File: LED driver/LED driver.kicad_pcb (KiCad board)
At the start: 2 copper layers, 50 x 40 mm, 42 parts, among them J1 Conn_VCC, J2 Conn_LED, J3 Conn_Aux, J4 Conn_UART, Q1 ZXMN3A01F, Q2 ZXMN3A01F, Q3 ZXMN3A01F, Q4 ZXMN3A01F, Q5 ZXMN3A01F, SW1 SW_Push, U1 ESP32-C3-MINI-1-N4, U2 MP2359

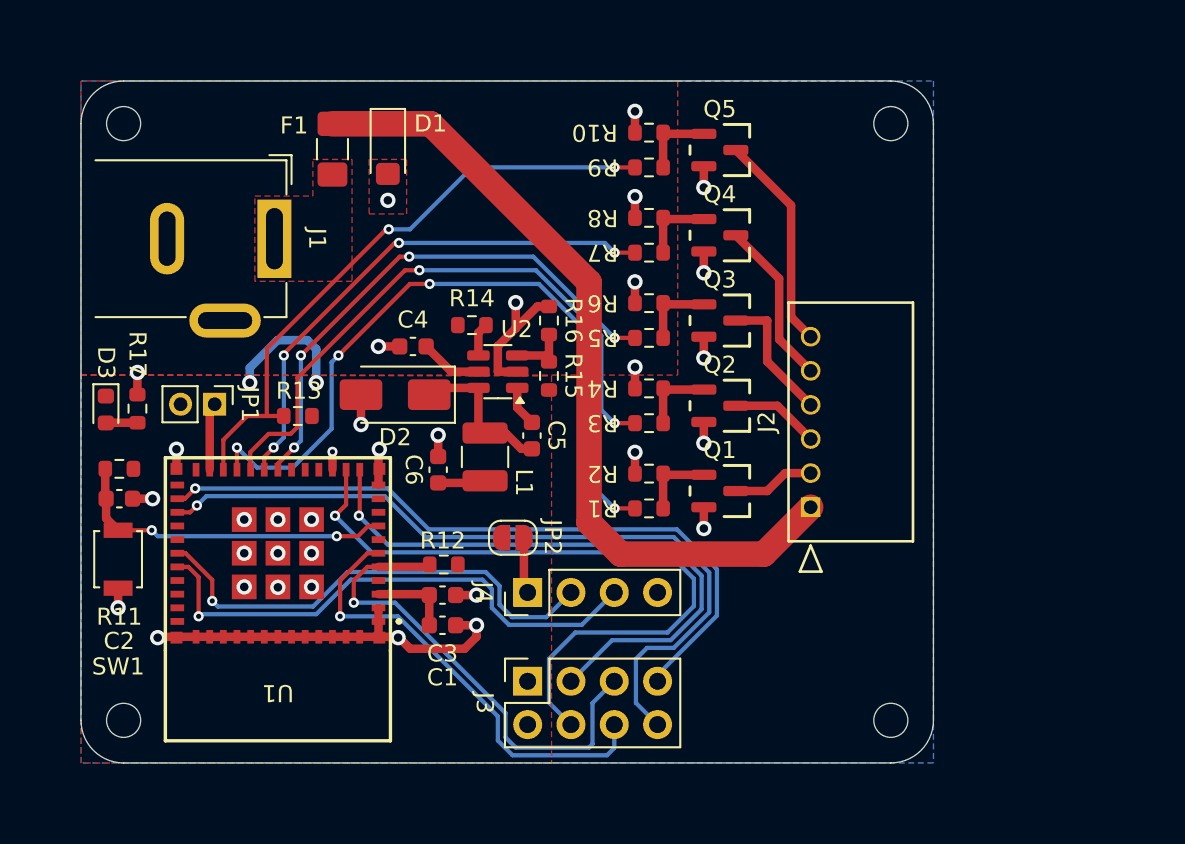
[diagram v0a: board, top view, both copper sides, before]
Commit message: 2024-06-04 002
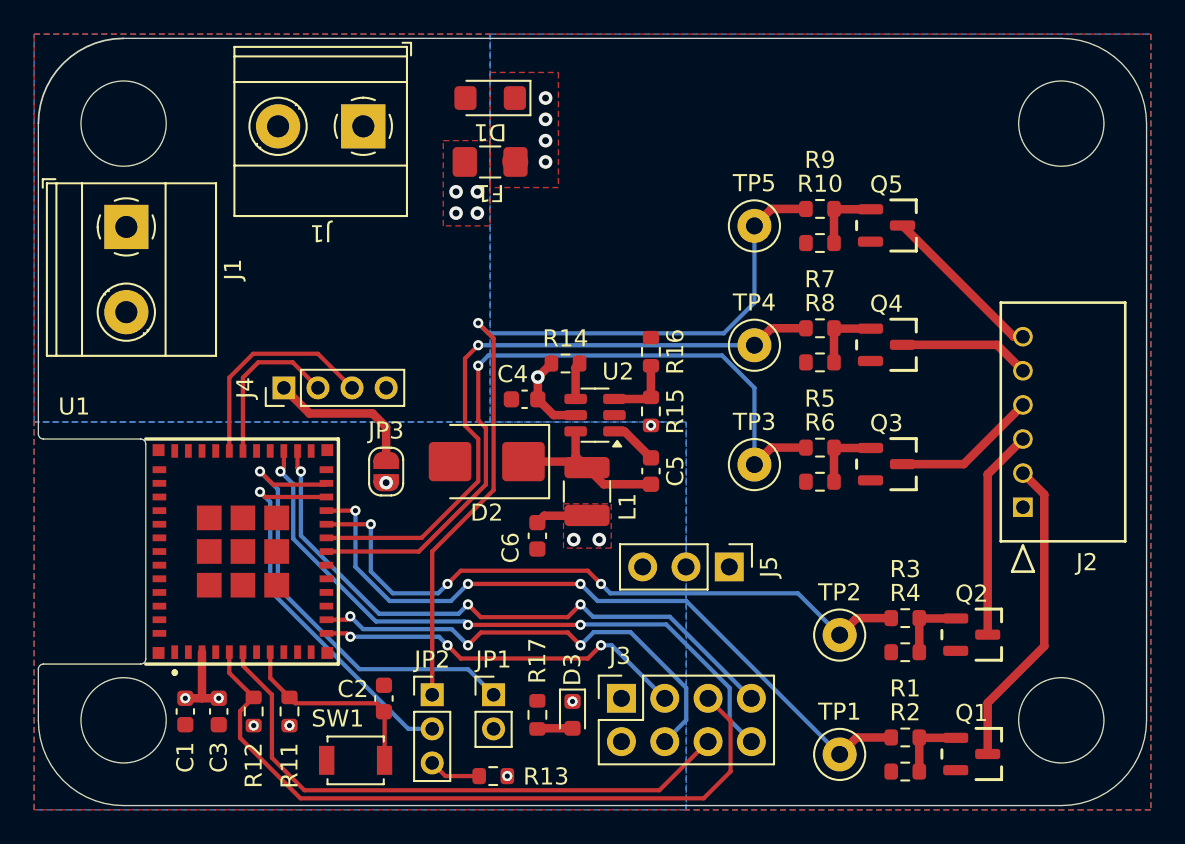
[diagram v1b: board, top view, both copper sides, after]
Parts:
- removed the J1 at (108.7, 64.3)
- added J1: Conn_VCC, TerminalBlock_Phoenix:TerminalBlock_Phoenix_MKDS-1,5-2_1x02_P5.00mm_Horizontal, F.Cu at (113.9, 57.7)
- added J1: Conn_VCC, TerminalBlock_Phoenix:TerminalBlock_Phoenix_MKDS-1,5-2_1x02_P5.00mm_Horizontal, F.Cu at (100.0, 63.6)
- added J5: PWR_AUX, Connector_PinHeader_2.54mm:PinHeader_1x03_P2.54mm_Vertical, F.Cu at (135.3, 83.6)
- added JP3: SolderJumper_2_Open, Jumper:SolderJumper-2_P1.3mm_Open_RoundedPad1.0x1.5mm, F.Cu at (115.2, 78.0)
- added TP1: PWM_W, TestPoint:TestPoint_Loop_D2.50mm_Drill1.0mm, F.Cu at (141.8, 94.6)
- added TP2: PWM_B, TestPoint:TestPoint_Loop_D2.50mm_Drill1.0mm, F.Cu at (141.8, 87.6)
- added TP3: PWM_R, TestPoint:TestPoint_Loop_D2.50mm_Drill1.0mm, F.Cu at (136.8, 77.6)
- added TP4: PWM_G, TestPoint:TestPoint_Loop_D2.50mm_Drill1.0mm, F.Cu at (136.8, 70.6)
- added TP5: PWM_WW, TestPoint:TestPoint_Loop_D2.50mm_Drill1.0mm, F.Cu at (136.8, 63.6)
- D2: value B230A -> B230-13-F; footprint Diode_SMD:D_SMA -> Diode_SMD:D_SMB
- J4: footprint Connector_PinHeader_2.54mm:PinHeader_1x04_P2.54mm_Vertical -> Connector_PinHeader_2.00mm:PinHeader_1x04_P2.00mm_Vertical
- JP1: value Boot_Mode -> Boot Mode 1
- JP2: value SolderJumper_2_Open -> Boot Mode 2; footprint Jumper:SolderJumper-2_P1.3mm_Open_RoundedPad1.0x1.5mm -> Connector_PinHeader_2.00mm:PinHeader_1x03_P2.00mm_Vertical
- R13: value 100K -> 4.7K
- moved D3 32.7 mm to (126.1, 92.3)
- moved R17 29.5 mm to (124.1, 92.3)
- moved R13 24.0 mm to (121.5, 95.8)
- moved JP1 23.6 mm to (121.5, 91.1), turned to 0 degrees
- moved R2 23.0 mm to (145.7, 95.6)
- moved R4 21.6 mm to (145.7, 88.6)
- moved Q1 21.4 mm to (149.6, 94.5)
- moved R1 20.2 mm to (145.7, 93.6)
- moved Q2 20.0 mm to (149.6, 87.5)
- moved C2 19.4 mm to (115.1, 91.3), turned to -90 degrees
- moved R3 18.9 mm to (145.7, 86.6)
- moved J4 18.7 mm to (109.2, 73.1)
- moved SW1 18.3 mm to (113.4, 94.9), turned to 0 degrees
- moved R11 17.4 mm to (109.5, 92.1), turned to 90 degrees
- moved C1 15.9 mm to (103.4, 92.1), turned to 90 degrees
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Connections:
- JP2 pad 1: +3.3V -> /PWM_WW
- JP2 pad 2: Net-(J4-Pin_1) -> Net-(JP2-C)
- R13 pad 2: /PWM_WW -> Net-(JP2-B)
- U1 pad 10: unconnected-(U1-NC_4-Pad10) -> (no net)
- U1 pad 15: unconnected-(U1-NC_5-Pad15) -> (no net)
- U1 pad 17: unconnected-(U1-NC_6-Pad17) -> (no net)
- U1 pad 22: /PWM_WW -> Net-(JP2-C)
- U1 pad 24: unconnected-(U1-NC_7-Pad24) -> (no net)
- U1 pad 25: unconnected-(U1-NC_8-Pad25) -> (no net)
- U1 pad 28: unconnected-(U1-NC_9-Pad28) -> (no net)
- U1 pad 29: unconnected-(U1-NC_10-Pad29) -> (no net)
- U1 pad 32: unconnected-(U1-NC_11-Pad32) -> (no net)
- U1 pad 33: unconnected-(U1-NC_12-Pad33) -> (no net)
- U1 pad 34: unconnected-(U1-NC_13-Pad34) -> (no net)
- U1 pad 35: unconnected-(U1-NC_14-Pad35) -> (no net)
- U1 pad 4: unconnected-(U1-NC_1-Pad4) -> (no net)
- U1 pad 7: unconnected-(U1-NC_2-Pad7) -> (no net)
- U1 pad 9: unconnected-(U1-NC_3-Pad9) -> (no net)
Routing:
- net GND: track 57.0 -> 0.00 mm, vias 34 -> 0
- net VCC: track 51.6 -> 5.09 mm, vias 0 -> 5
- net Net-(JP2-C): track 0.00 -> 22.9 mm, vias 0 -> 1
- net /IO9: track 3.96 -> 26.8 mm, vias 0 -> 1
- net /TX: track 31.6 -> 12.9 mm, vias 1 -> 0
- net /RX: track 28.3 -> 9.76 mm, vias 1 -> 0
- net /IO0: track 35.7 -> 22.1 mm, vias 1 -> 3
- net /W: track 4.83 -> 18.4 mm
- net /IO1: track 41.3 -> 27.9 mm, vias 1 -> 3
- net /PWM_WW: track 35.8 -> 48.8 mm, vias 2 -> 1
- net /IO2: track 28.8 -> 41.7 mm, vias 1 -> 0
- net /PWM_R: track 31.2 -> 43.3 mm, vias 4 -> 1
- net +3.3V: track 15.2 -> 7.06 mm, vias 2 -> 10
- net /PWM_G: track 30.8 -> 38.5 mm, vias 4 -> 1
- net Net-(U1-EN): track 19.6 -> 11.9 mm, vias 2 -> 0
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- added copper zone on B.Cu, net +3.3V
- added copper zone on B.Cu, net Net-(J1-Pin_2)
- added copper zone on B.Cu, net VCC
- removed copper zone on B.Cu, net GND
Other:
- board size 50 x 40 mm -> 65 x 45 mm
